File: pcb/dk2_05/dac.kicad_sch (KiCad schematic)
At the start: 34 parts, among them U13 TL072, U14 PCM5102

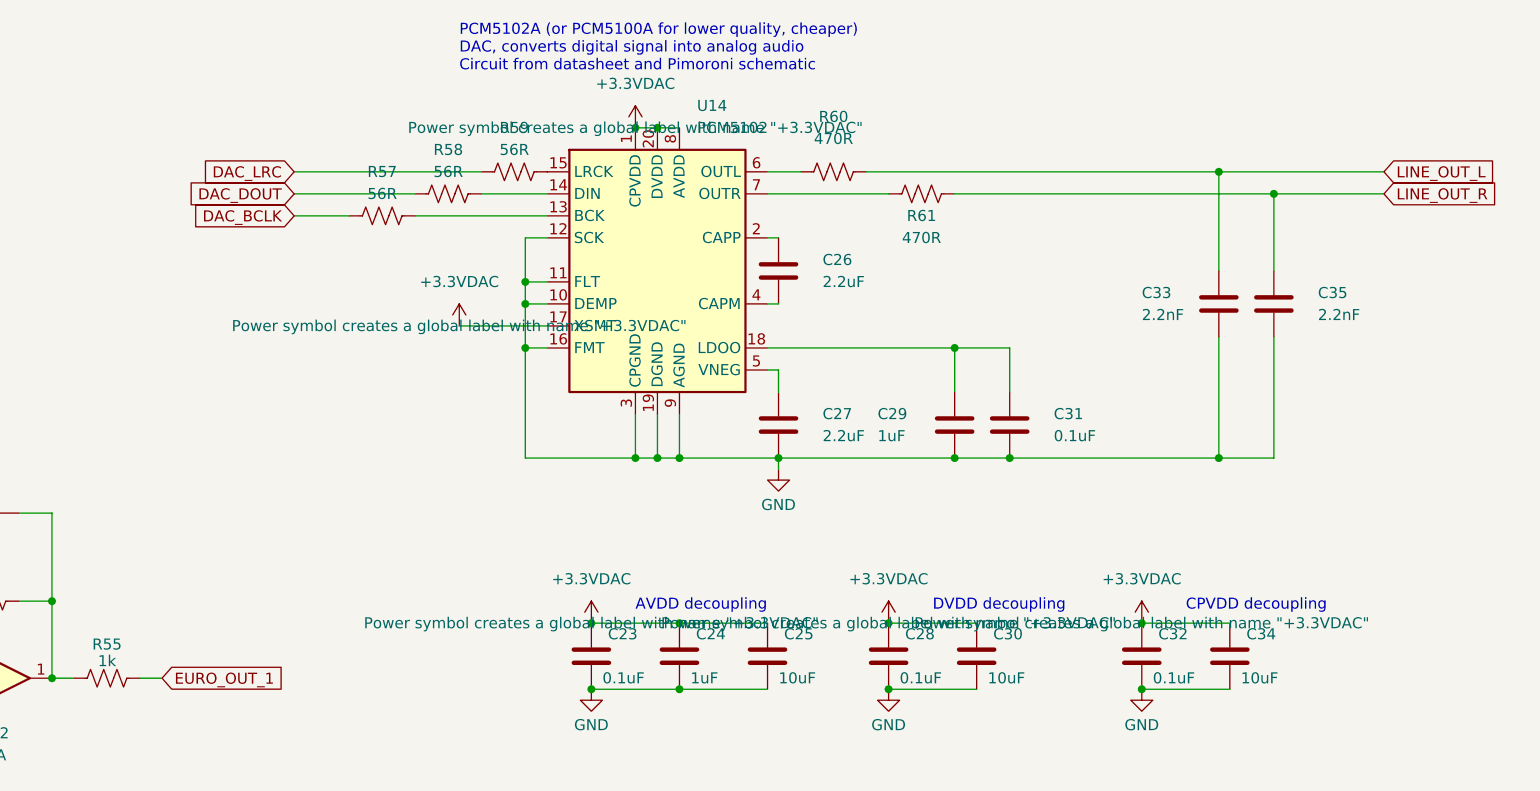
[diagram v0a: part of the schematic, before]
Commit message: all this layout stuff better be worth it
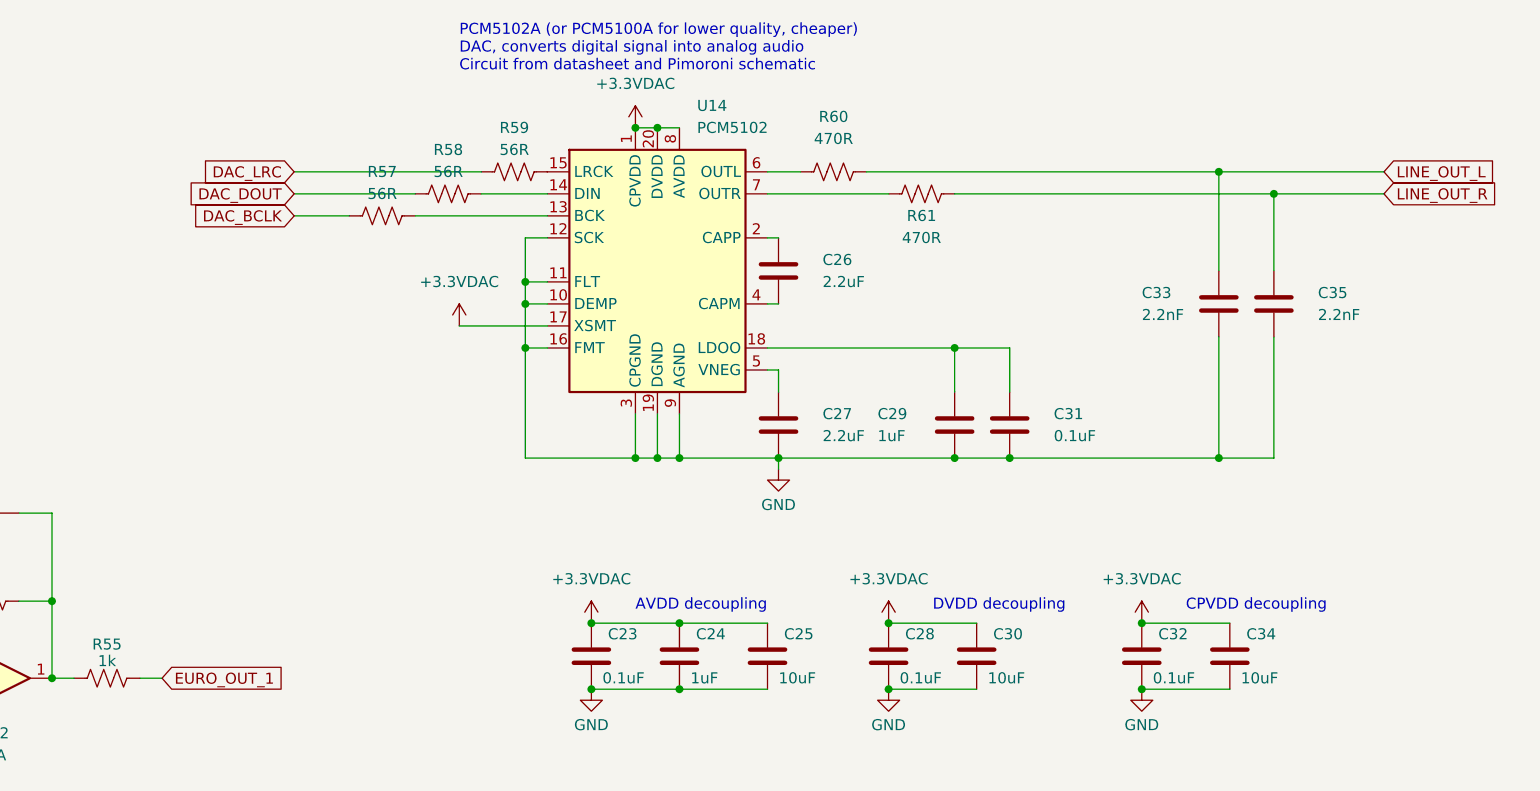
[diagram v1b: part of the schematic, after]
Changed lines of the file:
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@@
 					(size 1.27 1.27)
 				)
+				(hide yes)
 			)
 		)
@@
 					(size 1.27 1.27)
 				)
+				(hide yes)
 			)
 		)
@@
 					(size 1.27 1.27)
 				)
+				(hide yes)
 			)
 		)
@@
 					(size 1.27 1.27)
 				)
+				(hide yes)
 			)
 		)
@@
 					(size 1.27 1.27)
 				)
-			)
-		)
+				(hide yes)
+			)
+		)
